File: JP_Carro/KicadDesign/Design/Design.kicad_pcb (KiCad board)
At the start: 2 copper layers, 130.4 x 40 mm, 14 parts, among them J10 Puente_H2, J11 A MOTOR, J12 B MOTOR, J13 SENSOR_SOURCE, J5 SENSOR, J6 Conn_01x20_Socket, J7 Conn_01x20_Socket, J8 Puente H, J9 9V, U3.3V1 LM317_TO-220

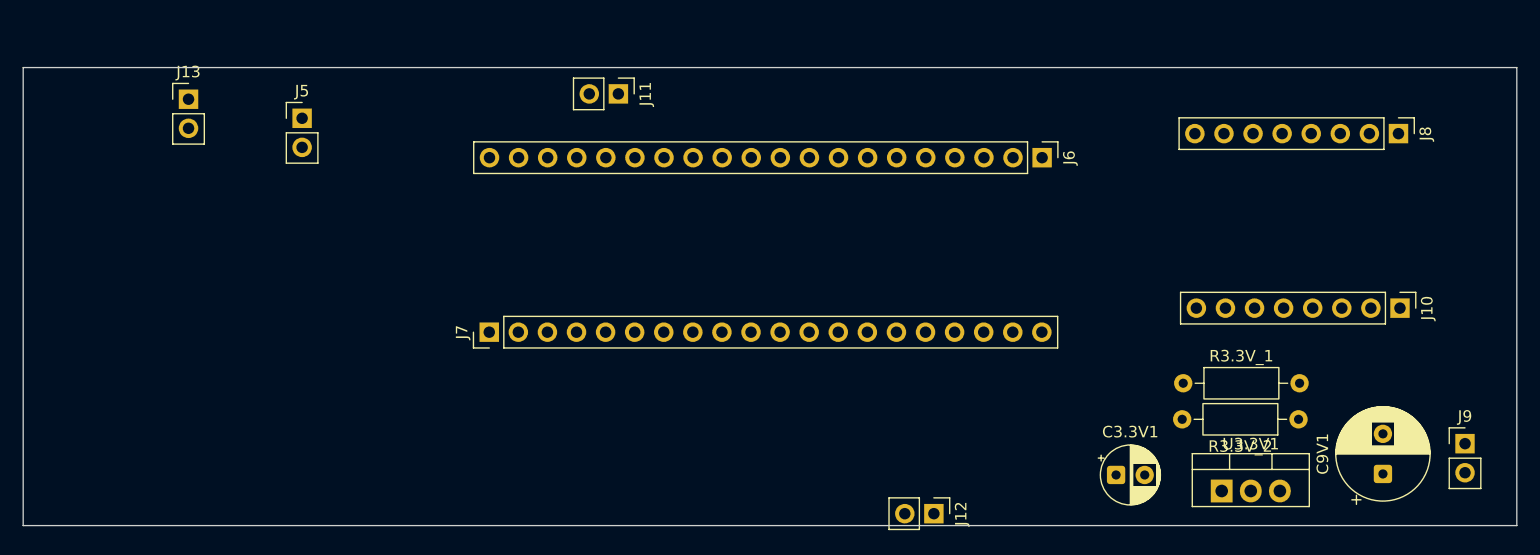
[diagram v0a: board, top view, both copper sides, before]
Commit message: Placa terminada
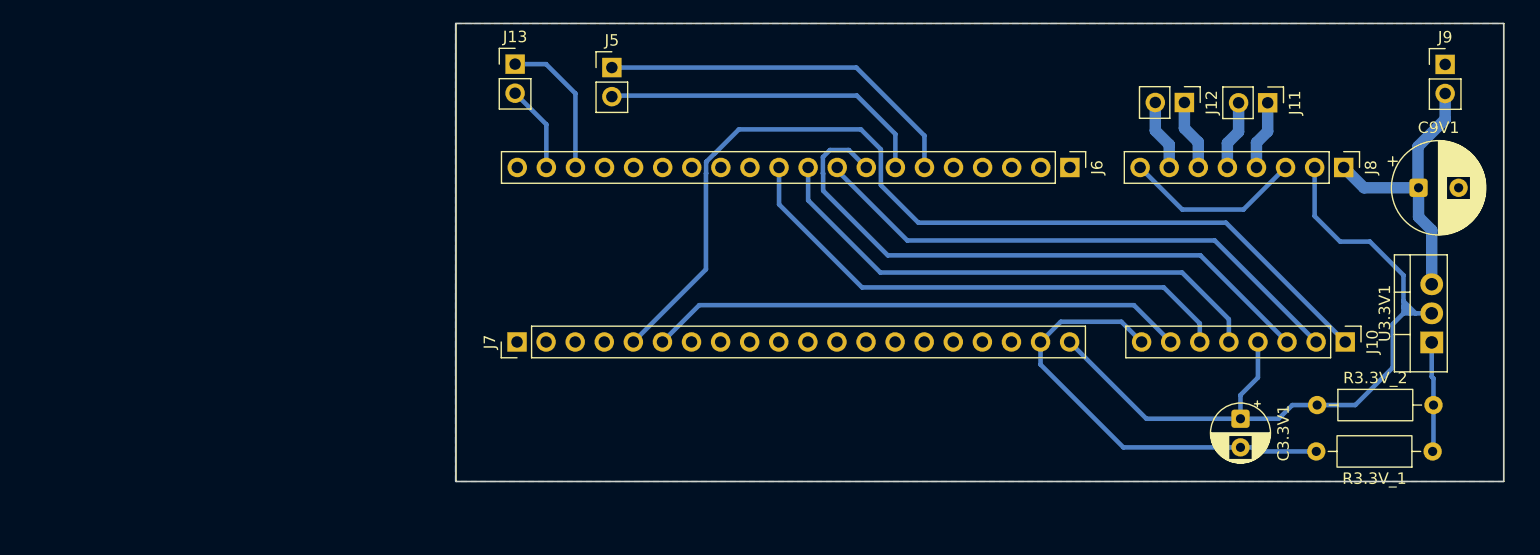
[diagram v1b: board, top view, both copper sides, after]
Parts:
- moved J11 56.7 mm to (147.6, 80.1)
- moved J12 42.0 mm to (140.3, 80.0)
- moved J9 33.2 mm to (163.1, 76.7)
- moved J13 28.7 mm to (81.8, 76.7)
- moved J5 27.4 mm to (90.3, 77.0)
- moved C9V1 25.2 mm to (160.8, 87.5), turned to 0 degrees
- moved R3.3V_1 22.6 mm to (162.0, 110.5), turned to 180 degrees
- moved U3.3V1 22.5 mm to (161.9, 101.0), turned to 90 degrees
- moved C3.3V1 11.9 mm to (145.2, 107.7), turned to -90 degrees
- moved J10 5.62 mm to (154.3, 101.0)
- moved J8 5.62 mm to (154.2, 85.7)
- moved J7 2.57 mm to (82.0, 101.0)
- moved J6 2.57 mm to (130.3, 85.7)
- moved R3.3V_2 2.05 mm to (151.9, 106.5), turned to 0 degrees
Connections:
- J7 pad 19: unconnected-(J7-Pin_19-Pad19) -> GND
- J7 pad 20: unconnected-(J7-Pin_20-Pad20) -> 3.3V
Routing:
- net A8 PWM_IZQ: track 0.00 -> 84.9 mm
- net 3.3V: track 0.00 -> 80.3 mm
- net GND: track 0.00 -> 62.8 mm
- net A2 AIN1: track 0.00 -> 53.6 mm
- net A3 AIN2: track 0.00 -> 48.3 mm
- net A9 PWM_DER: track 0.00 -> 47.1 mm
- net A5 BIN2: track 0.00 -> 45.9 mm
- net A4 BIN1: track 0.00 -> 45.9 mm
- net A0 ADC_1: track 0.00 -> 32.5 mm
- net A1 ADC_2: track 0.00 -> 29.1 mm
- net 9V: track 0.00 -> 25.3 mm
- net Net-(U3.3V1-ADJ): track 0.00 -> 9.62 mm
- net /B02: track 0.00 -> 6.18 mm
- net /B01: track 0.00 -> 6.18 mm
- net /A02: track 0.00 -> 6.06 mm
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- added copper zone on B.Cu, net GND
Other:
- board size 130.4 x 40 mm -> 91.5 x 40 mm
